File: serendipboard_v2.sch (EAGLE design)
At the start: 28 parts, among them IC1 TP4056, IC2 DW01A, Q1 FS8205A, Q2 DMP3056LSD, U1 MAX17043, U2 AP2112-3.3, U3 AP2112-3.3

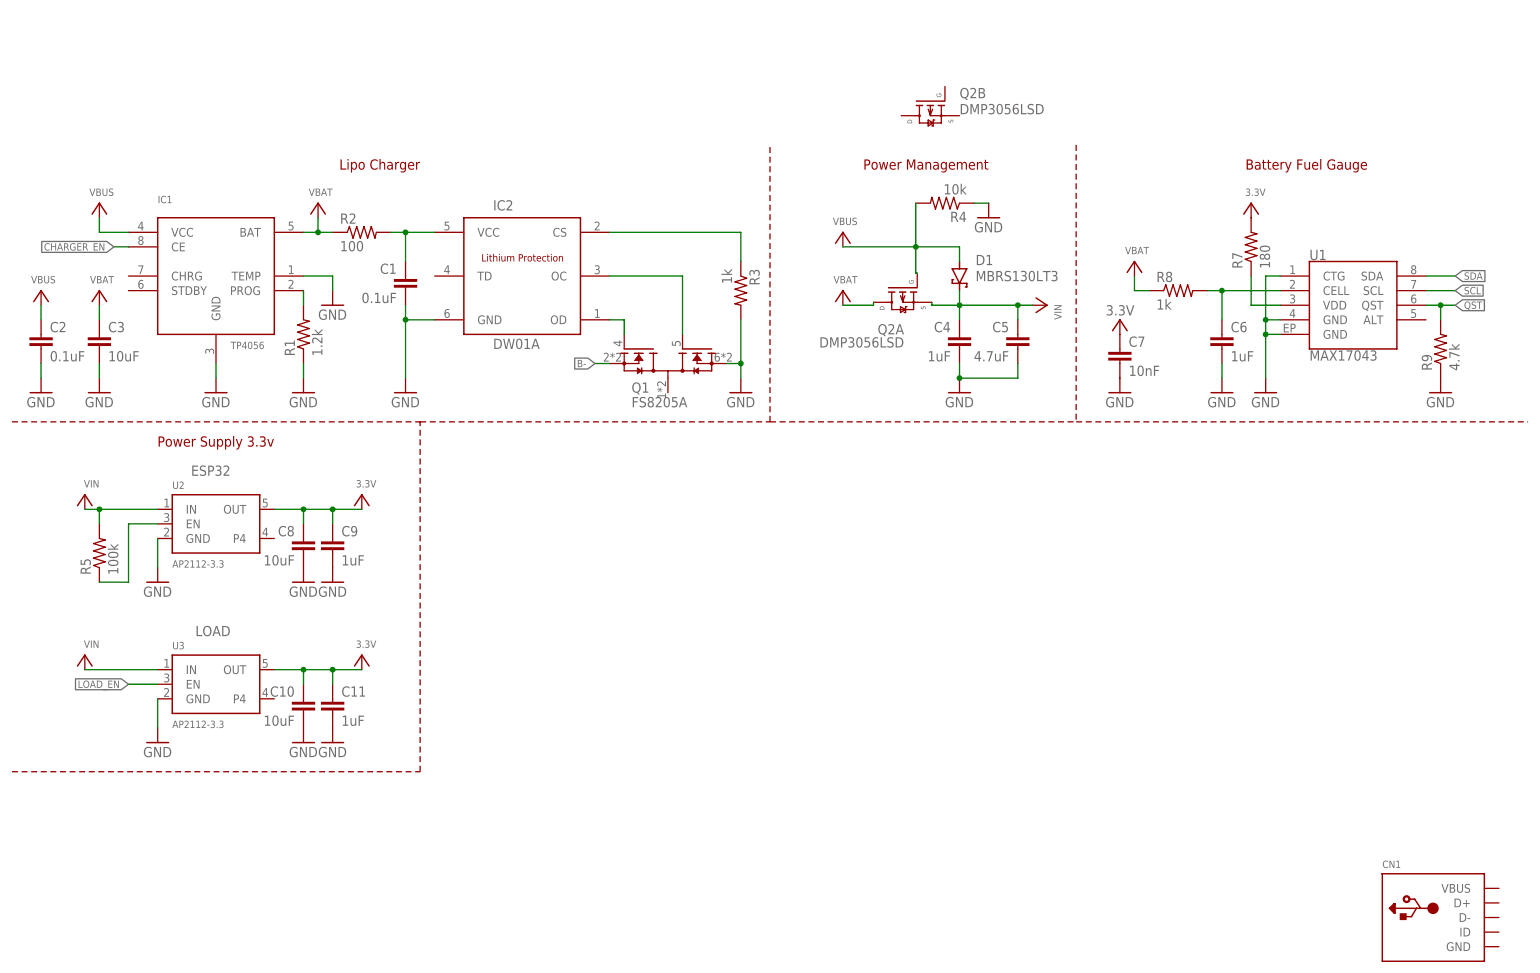
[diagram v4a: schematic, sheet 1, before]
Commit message: Update serendipboard_v2.sch
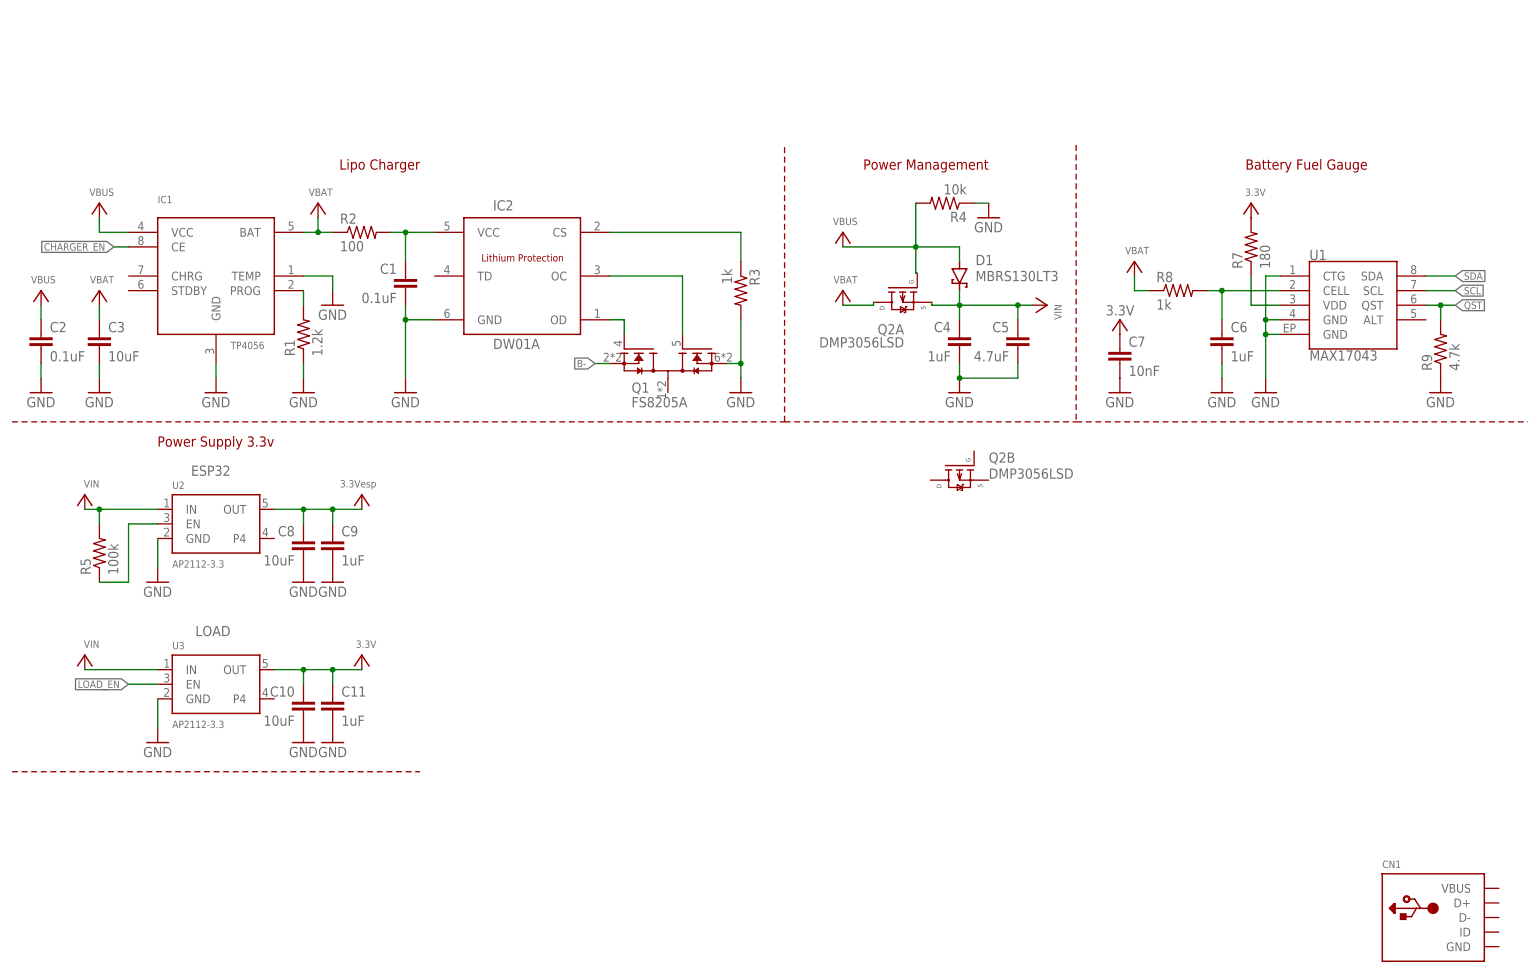
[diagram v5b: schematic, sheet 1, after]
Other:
- moved on the sheet: Q2B
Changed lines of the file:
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@@
 <part name="GND15" library="supply1" library_urn="urn:adsk.eagle:library:371" deviceset="GND" device=""/>
 <part name="GND16" library="supply1" library_urn="urn:adsk.eagle:library:371" deviceset="GND" device=""/>
-<part name="P+8" library="supply1" library_urn="urn:adsk.eagle:library:371" deviceset="VCC" device="" value="3.3V"/>
+<part name="P+8" library="supply1" library_urn="urn:adsk.eagle:library:371" deviceset="VCC" device="" value="3.3Vesp"/>
 <part name="U3" library="microbuilder" deviceset="VREG_SOT23-5" device="" value="AP2112-3.3"/>
 <part name="C10" library="rcl" library_urn="urn:adsk.eagle:library:334" deviceset="C-EU" device="C0805" package3d_urn="urn:adsk.eagle:package:23617/2" value="10uF"/>
@@
 <plain>
 <text x="71.12" y="177.8" size="1.778" layer="94" rot="R180">Lipo Charger</text>
-<wire x1="0" y1="132.08" x2="71.12" y2="132.08" width="0.1524" layer="94" style="shortdash"/>
-<wire x1="71.12" y1="132.08" x2="132.08" y2="132.08" width="0.1524" layer="94" style="shortdash"/>
-<wire x1="132.08" y1="132.08" x2="132.08" y2="180.34" width="0.1524" layer="94" style="shortdash"/>
-<wire x1="132.08" y1="132.08" x2="185.42" y2="132.08" width="0.1524" layer="94" style="shortdash"/>
+<wire x1="0" y1="132.08" x2="134.62" y2="132.08" width="0.1524" layer="94" style="shortdash"/>
+<wire x1="134.62" y1="132.08" x2="134.62" y2="180.34" width="0.1524" layer="94" style="shortdash"/>
+<wire x1="134.62" y1="132.08" x2="185.42" y2="132.08" width="0.1524" layer="94" style="shortdash"/>
 <text x="170.18" y="177.8" size="1.778" layer="94" rot="R180">Power Management</text>
 <wire x1="185.42" y1="132.08" x2="264.16" y2="132.08" width="0.1524" layer="94" style="shortdash"/>
@@
 <text x="38.1" y="96.52" size="1.778" layer="95" rot="R180">LOAD</text>
 <wire x1="0" y1="71.12" x2="71.12" y2="71.12" width="0.1524" layer="94" style="shortdash"/>
-<wire x1="71.12" y1="71.12" x2="71.12" y2="132.08" width="0.1524" layer="94" style="shortdash"/>
 </plain>
 <instances>
@@
 <attribute name="NAME" x="155.448" y="149.098" size="1.778" layer="95" rot="R180"/>
 </instance>
-<instance part="Q2" gate="B" x="160.02" y="187.96" smashed="yes" rot="R270">
-<attribute name="VALUE" x="165.1" y="187.452" size="1.778" layer="96" align="top-left"/>
-<attribute name="NAME" x="165.1" y="188.468" size="1.778" layer="95"/>
+<instance part="Q2" gate="B" x="165.1" y="124.46" smashed="yes" rot="R270">
+<attribute name="VALUE" x="170.18" y="123.952" size="1.778" layer="96" align="top-left"/>
+<attribute name="NAME" x="170.18" y="124.968" size="1.778" layer="95"/>
 </instance>
 <instance part="R4" gate="G$1" x="162.56" y="170.18" smashed="yes" rot="R180">

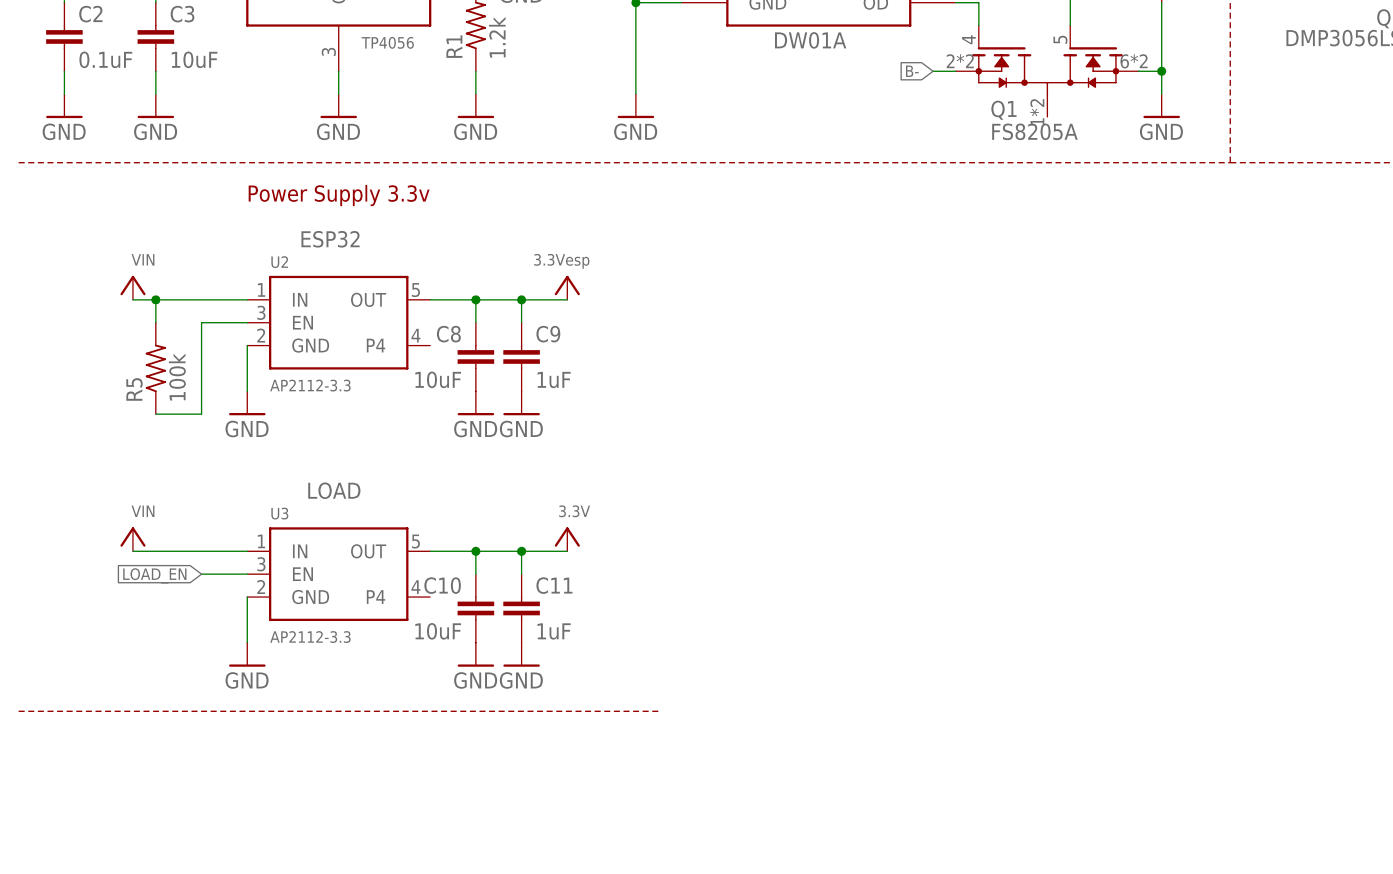
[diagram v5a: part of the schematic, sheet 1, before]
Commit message: Update serendipboard_v2.sch
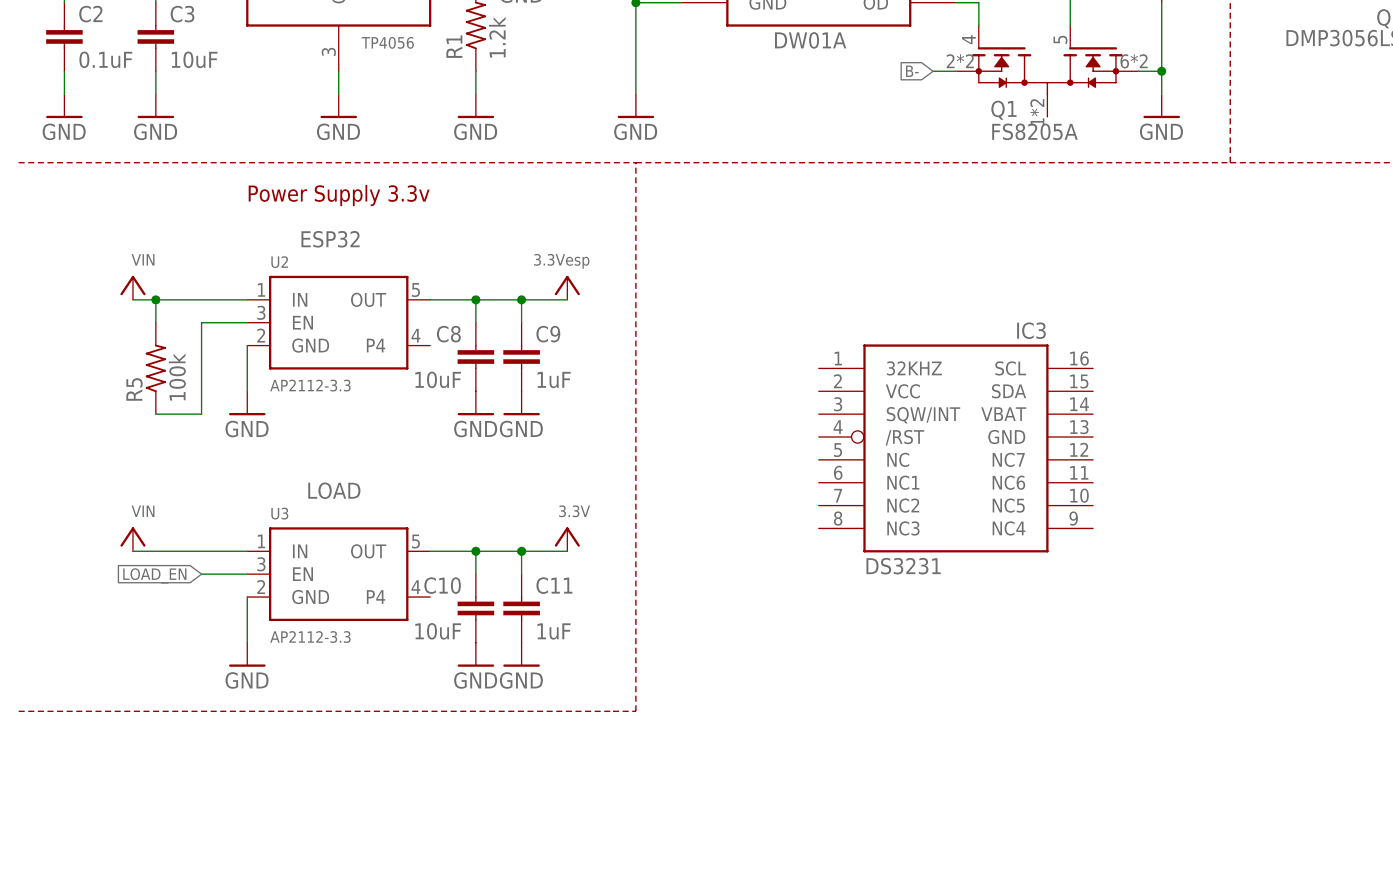
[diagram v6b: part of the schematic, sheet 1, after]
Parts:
- added IC3: DS3231/SO, DS3231:DS3231/SO
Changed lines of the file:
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@@
 <part name="P+10" library="supply1" library_urn="urn:adsk.eagle:library:371" deviceset="VCC" device="" value="VIN"/>
 <part name="P+11" library="supply1" library_urn="urn:adsk.eagle:library:371" deviceset="VCC" device="" value="3.3V"/>
+<part name="IC3" library="DS3231" deviceset="DS3231" device="/SO"/>
 </parts>
 <sheets>
@@
 <plain>
 <text x="71.12" y="177.8" size="1.778" layer="94" rot="R180">Lipo Charger</text>
-<wire x1="0" y1="132.08" x2="134.62" y2="132.08" width="0.1524" layer="94" style="shortdash"/>
+<wire x1="0" y1="132.08" x2="68.58" y2="132.08" width="0.1524" layer="94" style="shortdash"/>
+<wire x1="68.58" y1="132.08" x2="134.62" y2="132.08" width="0.1524" layer="94" style="shortdash"/>
 <wire x1="134.62" y1="132.08" x2="134.62" y2="180.34" width="0.1524" layer="94" style="shortdash"/>
 <wire x1="134.62" y1="132.08" x2="185.42" y2="132.08" width="0.1524" layer="94" style="shortdash"/>
@@
 <text x="38.1" y="124.46" size="1.778" layer="95" rot="R180">ESP32</text>
 <text x="38.1" y="96.52" size="1.778" layer="95" rot="R180">LOAD</text>
-<wire x1="0" y1="71.12" x2="71.12" y2="71.12" width="0.1524" layer="94" style="shortdash"/>
+<wire x1="0" y1="71.12" x2="66.04" y2="71.12" width="0.1524" layer="94" style="shortdash"/>
+<wire x1="66.04" y1="71.12" x2="68.58" y2="71.12" width="0.1524" layer="94" style="shortdash"/>
+<wire x1="68.58" y1="71.12" x2="68.58" y2="132.08" width="0.1524" layer="94" style="shortdash"/>
 </plain>
 <instances>
@@
 <attribute name="VALUE" x="63.5" y="93.98" size="1.27" layer="96" rot="R180"/>
 </instance>
+<instance part="IC3" gate="G$1" x="104.14" y="99.06" smashed="yes">
+<attribute name="NAME" x="114.3" y="114.3" size="1.778" layer="95" rot="R180"/>
+</instance>
 </instances>
